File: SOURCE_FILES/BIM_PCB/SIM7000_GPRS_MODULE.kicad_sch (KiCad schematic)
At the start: 49 parts, among them J5 SIM_Card, Q5 BSN20, U2 SIM7000G

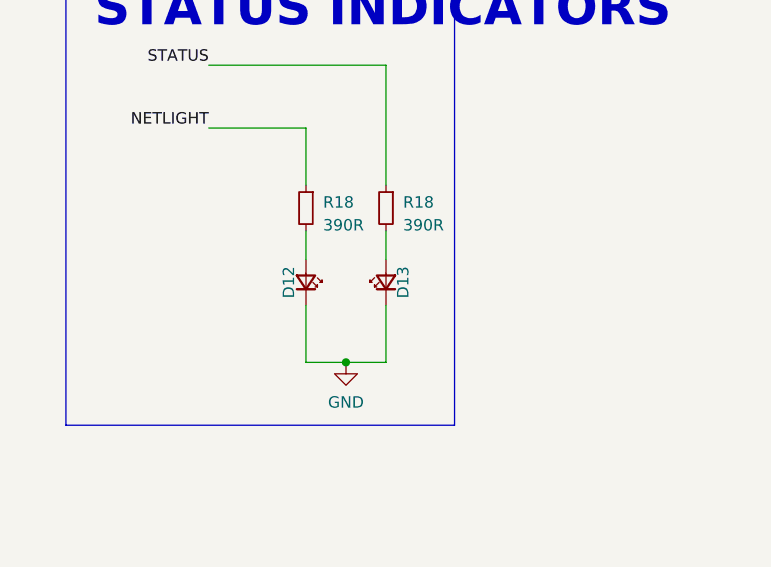
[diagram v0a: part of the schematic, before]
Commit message: updates on schematic and complete layout
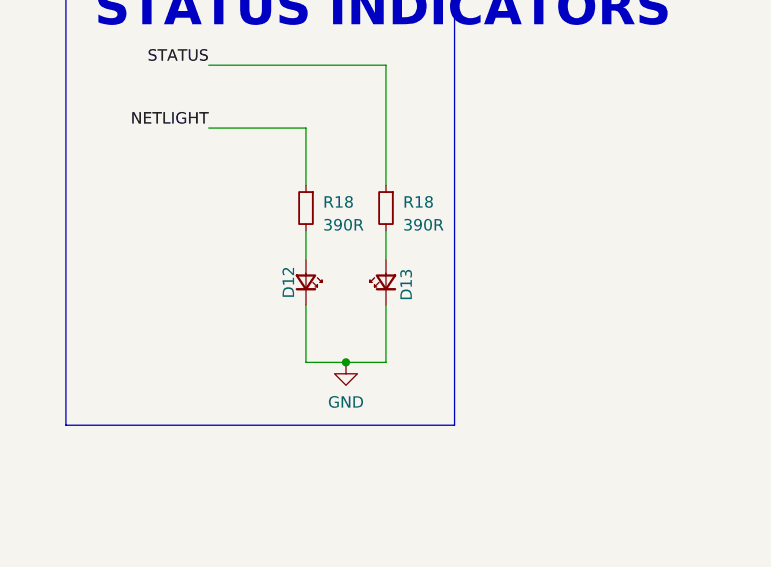
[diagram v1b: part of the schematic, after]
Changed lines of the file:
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@@
   (symbol (lib_id "Device:LED_Small") (at 276.225 149.225 90) (unit 1)
     (in_bom yes) (on_board yes) (dnp no)
-    (property "Reference" "D13" (at 278.13 149.225 0)
+    (property "Reference" "D13" (at 278.511 149.479 0)
       (effects (font (size 1.27 1.27)))
     )
